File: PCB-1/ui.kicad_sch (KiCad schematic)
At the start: 67 parts, among them Q1 BSD235C, Q2 PJC7407_R1, U10 NavigationSwitch_JS1400, U12 74AHCV17A, U15 150060RV75240, U16 150060RV75240, U7 OLED-1.5-SSD1327, U9 TLV61046ADB

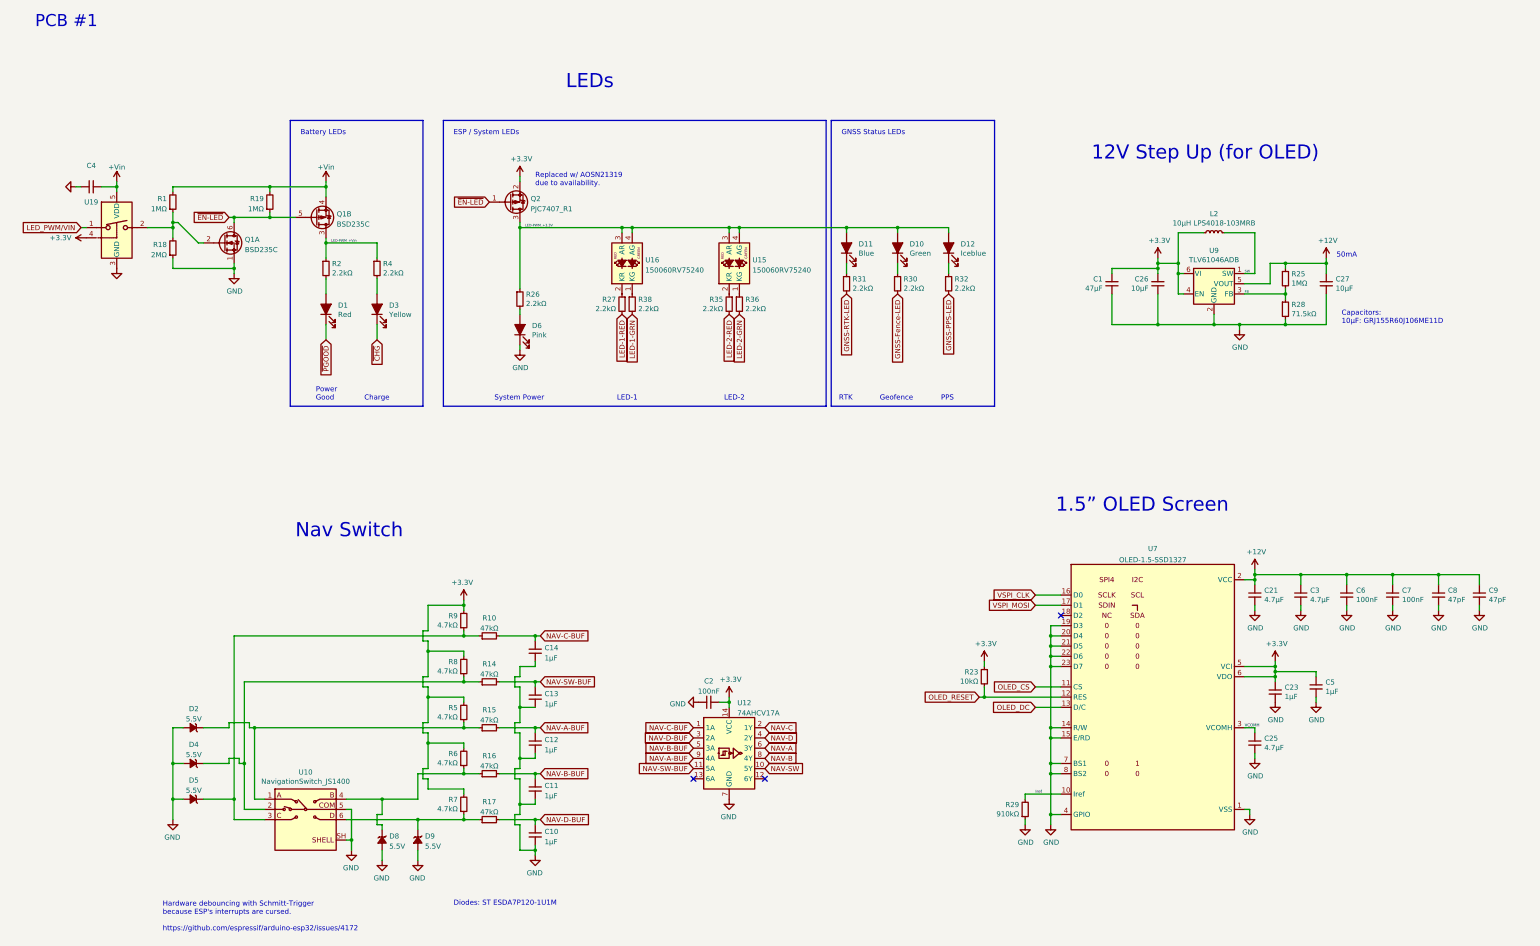
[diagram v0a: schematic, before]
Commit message: added photos to docu
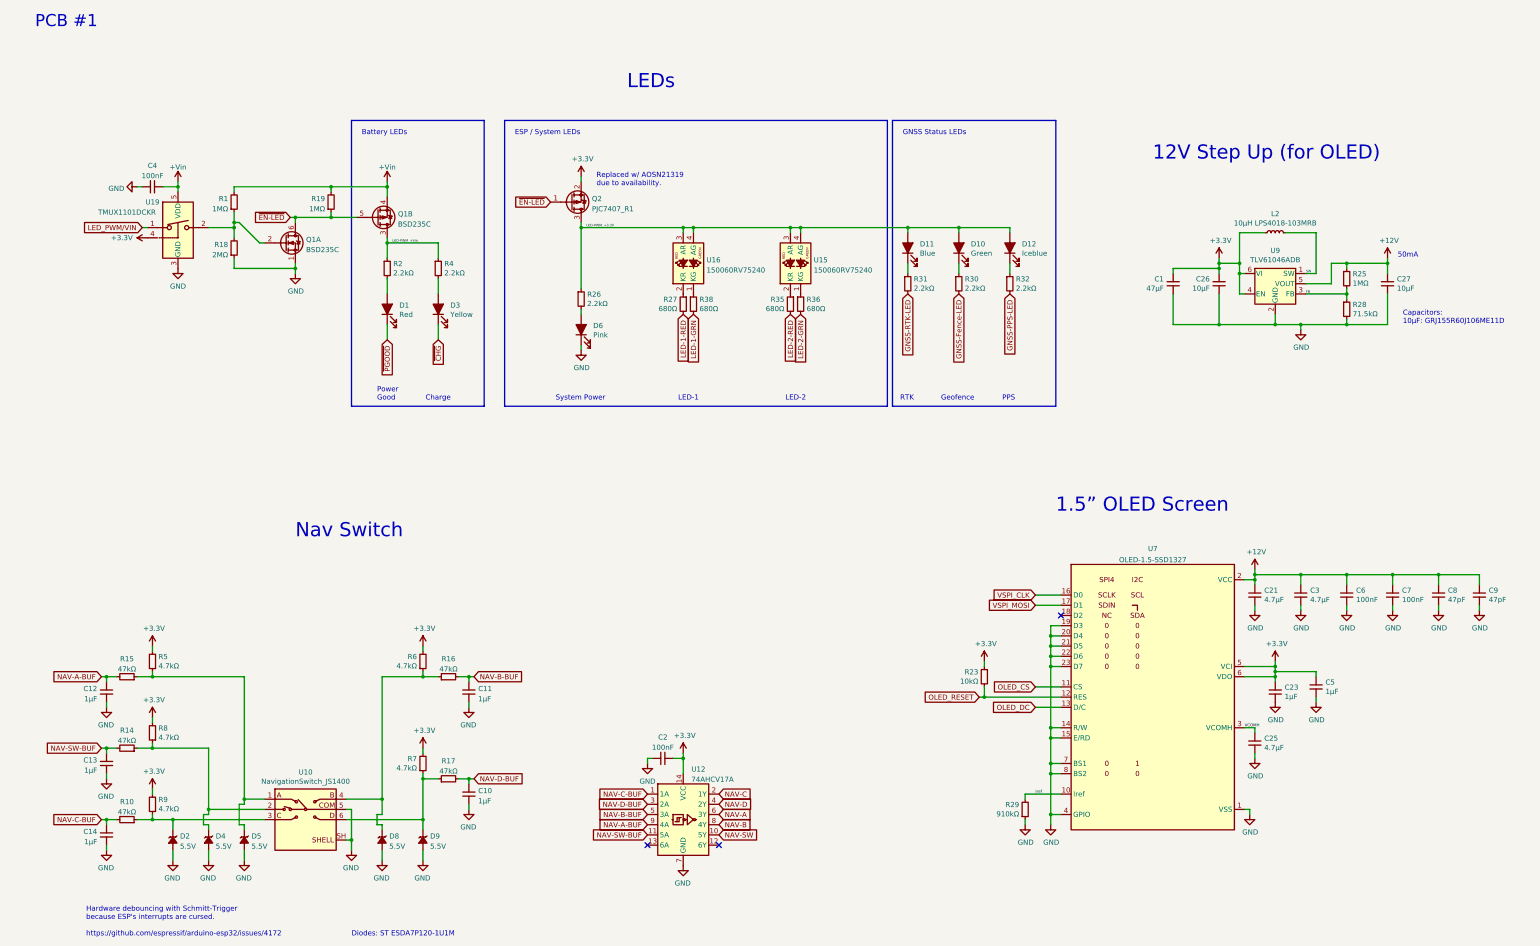
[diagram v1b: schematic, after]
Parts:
- C4: value (none) -> 100nF; footprint (none) -> Franz-Lib:C_0402_1005Metric_NoSilk
- R27, R35, R36, R38: value 2.2kΩ -> 680Ω
- U19: value (none) -> TMUX1101DCKR; footprint (none) -> Franz-Lib:Texas_SC70_(DCK)_NoSilk
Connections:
- net at R15.1, R5.1, U10.1 (A): now also D5.1 (K); no longer D2.1 (K)
- net at R10.1, R9.1, U10.3 (C): now also D2.1 (K); no longer D5.1 (K)
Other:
- moved on the sheet: C1, C10, C11, C12, C13, C14, C2, C26, C27, C4, D1, D10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
